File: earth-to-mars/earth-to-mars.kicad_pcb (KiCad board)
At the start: 2 copper layers, 36 x 40 mm, 12 parts, among them P7 CONN_01X06, P8 CONN_01X04, Q1 Q_NMOS_DGS, U1 mq8, U2 dht11

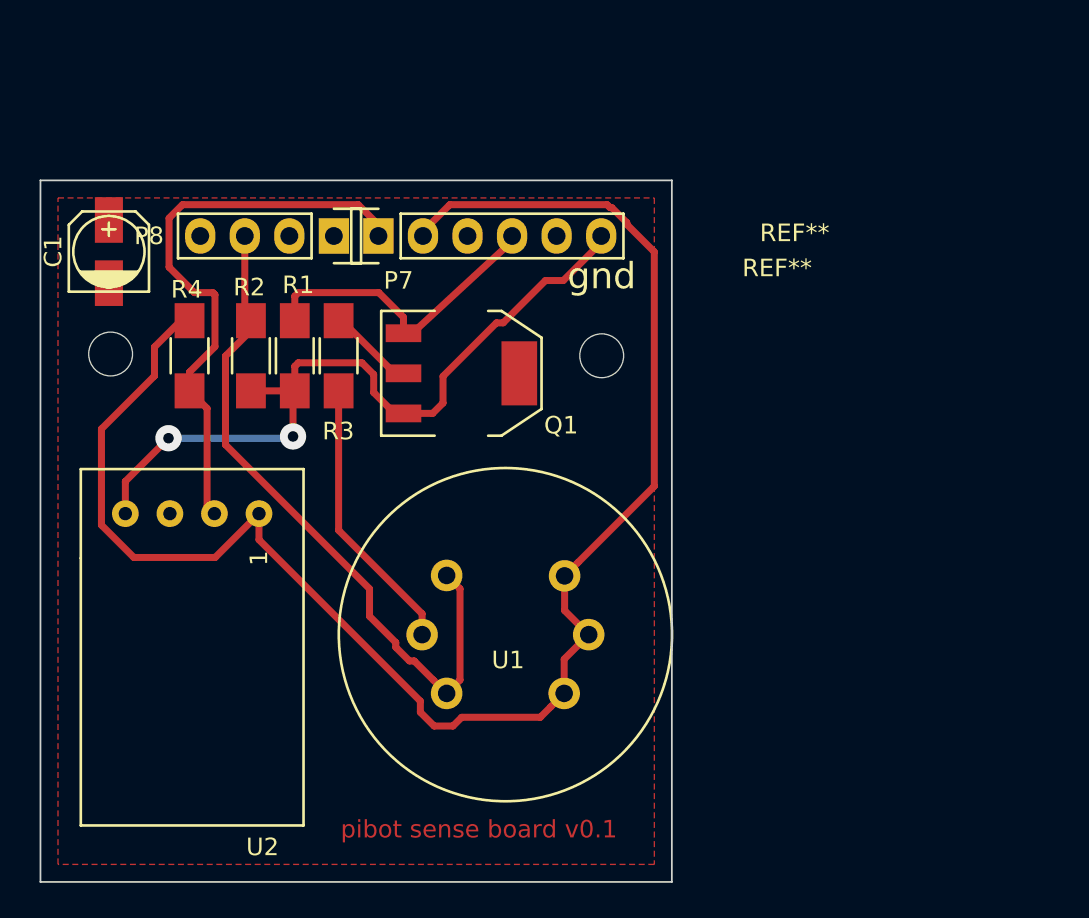
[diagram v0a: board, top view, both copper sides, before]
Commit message: mq8 sensor board
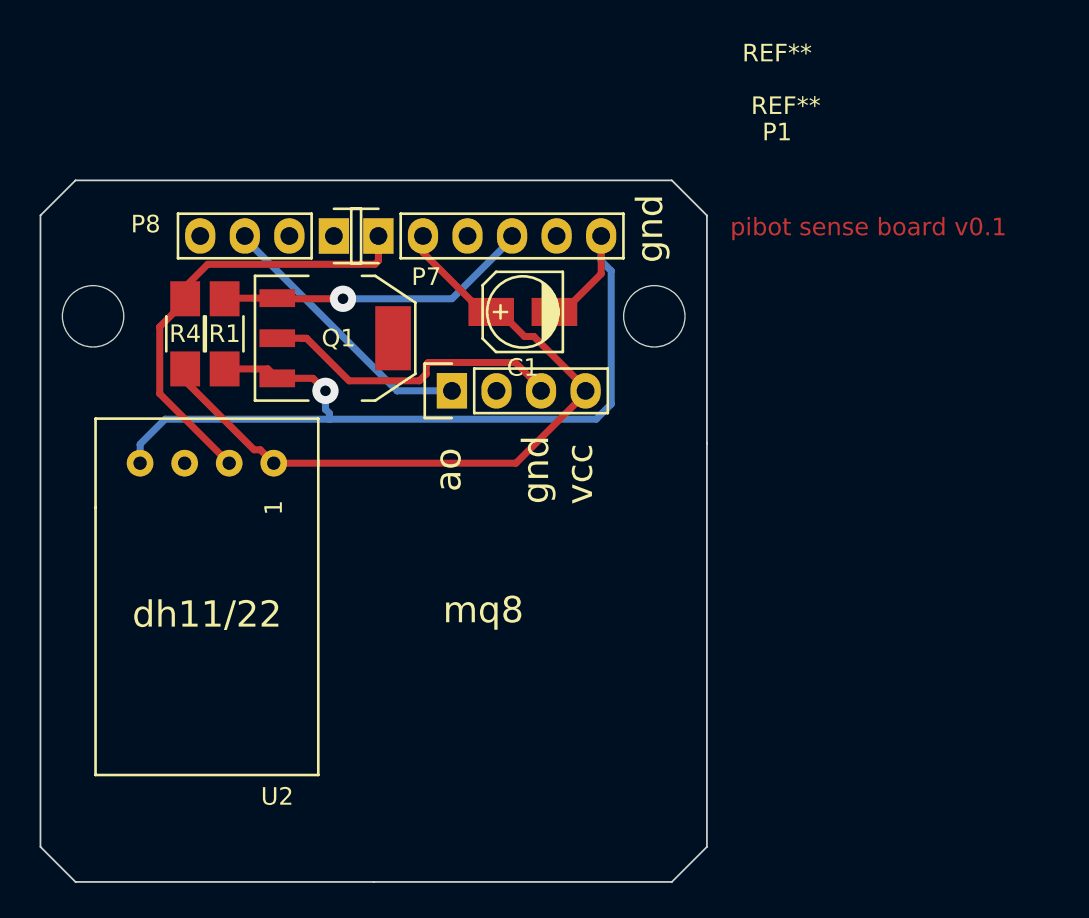
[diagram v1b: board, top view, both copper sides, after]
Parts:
- removed R2: 4.7k, Resistors_SMD:R_1206_HandSoldering
- removed R3: 5R, Resistors_SMD:R_1206_HandSoldering
- removed the REF** at (113.0, 96.9)
- removed the REF** at (141.0, 97.0)
- removed U1: mq8, fp:mq8
- added P1: CONN_01X04, Pin_Headers:Pin_Header_Straight_1x04, F.Cu at (132.5, 99.0)
- added REF**: MountingHole_3-5mm, Mounting_Holes:MountingHole_3-5mm, F.Cu at (144.0, 94.8)
- added REF**: MountingHole_3-5mm, Mounting_Holes:MountingHole_3-5mm, F.Cu at (112.0, 94.8)
- moved C1 23.8 mm to (136.5, 94.5), turned to 180 degrees
- moved Q1 7.47 mm to (125.8, 96.0)
- moved R1 4.19 mm to (119.5, 95.8)
- moved U2 3.00 mm to (112.1, 103.1)
- moved R4 1.27 mm to (117.2, 95.8), turned to 90 degrees
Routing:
- net +5V: track 92.9 -> 40.8 mm
- net mega_adc6: track 39.6 -> 15.6 mm
- net Net-(R3-Pad1): track 15.9 -> 0.00 mm
- net Net-(P1-Pad3): track 4.94 -> 17.5 mm
- net Earth: track 43.7 -> 52.4 mm, vias 2 -> 1
- net mega_io12_miso: track 33.1 -> 25.3 mm
- net mega_io11_mosi: track 17.7 -> 18.0 mm, vias 0 -> 1
- removed copper zone on F.Cu, net Earth
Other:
- board size 36 x 40 mm -> 38 x 40 mm
- board text added: "ao"
- board text added: "dh11/22"
- board text added: "mq8"
- board text added: "vcc"
